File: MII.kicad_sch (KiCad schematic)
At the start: 2 parts, among them U2 ICE40HX8K-BG121

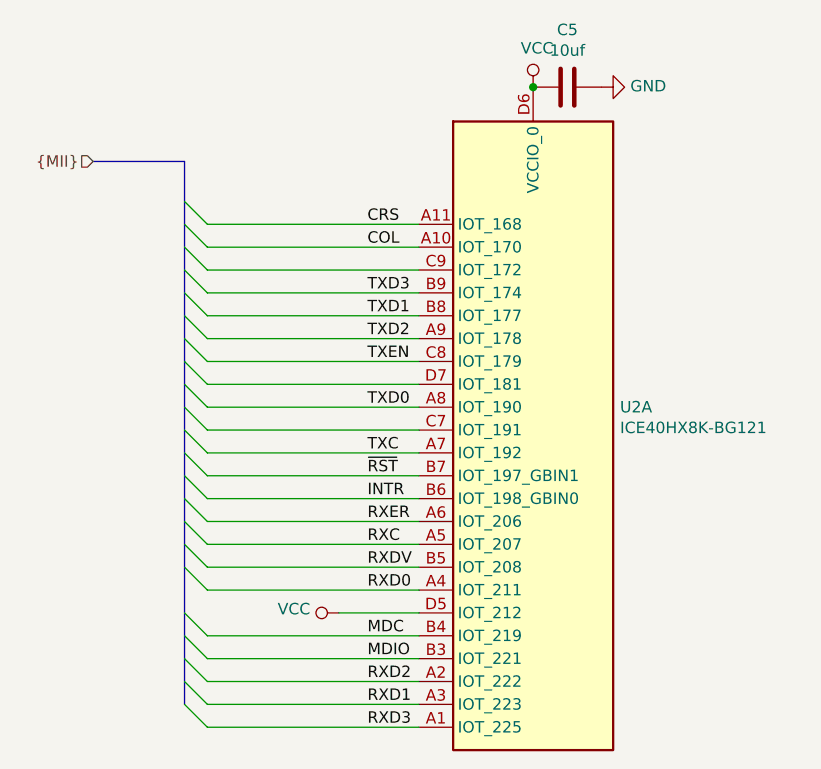
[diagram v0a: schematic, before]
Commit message: Routing changes, pullups, etc
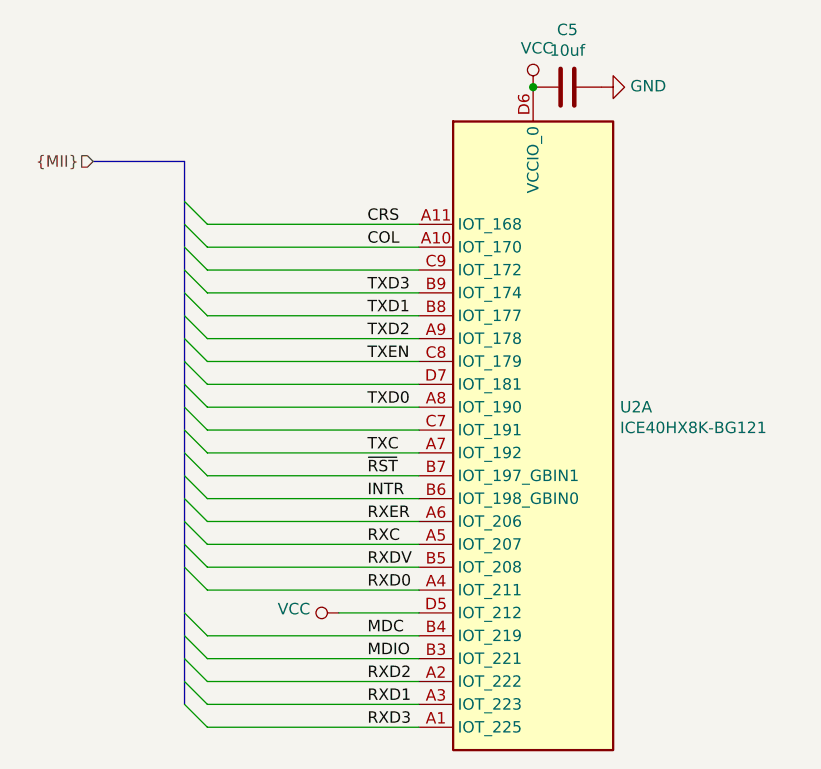
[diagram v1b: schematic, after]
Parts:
- C5, U2: Source (none) -> ANY
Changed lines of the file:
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@@
-(kicad_sch (version 20200512) (host eeschema "5.99.0-unknown-711fc99~101~ubuntu20.04.1")
-  (page 1 7)
+(kicad_sch (version 20200512) (host eeschema "5.99.0-unknown-eae0c14~101~ubuntu20.04.1")
+  (page 3 7)
   (paper "A4")
   (junction (at 111.125 62.23))
@@
   (bus_entry (at 72.39 128.27) (size 2.54 2.54))
   (bus_entry (at 72.39 130.81) (size 2.54 2.54))
-  (wire (pts (xy 74.93 77.47) (xy 98.425 77.47)))
-  (wire (pts (xy 74.93 80.01) (xy 98.425 80.01)))
-  (wire (pts (xy 74.93 82.55) (xy 98.425 82.55)))
-  (wire (pts (xy 74.93 85.09) (xy 98.425 85.09)))
-  (wire (pts (xy 74.93 87.63) (xy 98.425 87.63)))
-  (wire (pts (xy 74.93 90.17) (xy 98.425 90.17)))
-  (wire (pts (xy 74.93 92.71) (xy 98.425 92.71)))
-  (wire (pts (xy 74.93 95.25) (xy 98.425 95.25)))
-  (wire (pts (xy 74.93 97.79) (xy 98.425 97.79)))
-  (wire (pts (xy 74.93 100.33) (xy 98.425 100.33)))
-  (wire (pts (xy 74.93 102.87) (xy 98.425 102.87)))
-  (wire (pts (xy 74.93 105.41) (xy 98.425 105.41)))
-  (wire (pts (xy 74.93 107.95) (xy 98.425 107.95)))
-  (wire (pts (xy 74.93 110.49) (xy 98.425 110.49)))
-  (wire (pts (xy 74.93 113.03) (xy 98.425 113.03)))
-  (wire (pts (xy 74.93 115.57) (xy 98.425 115.57)))
-  (wire (pts (xy 74.93 118.11) (xy 98.425 118.11)))
-  (wire (pts (xy 74.93 123.19) (xy 98.425 123.19)))
-  (wire (pts (xy 74.93 125.73) (xy 98.425 125.73)))
-  (wire (pts (xy 74.93 128.27) (xy 98.425 128.27)))
-  (wire (pts (xy 74.93 130.81) (xy 98.425 130.81)))
-  (wire (pts (xy 74.93 133.35) (xy 98.425 133.35)))
-  (wire (pts (xy 89.535 120.65) (xy 98.425 120.65)))
-  (bus (pts (xy 62.23 70.485) (xy 72.39 70.485)))
-  (bus (pts (xy 72.39 70.485) (xy 72.39 77.47)))
-  (bus (pts (xy 72.39 77.47) (xy 72.39 82.55)))
-  (bus (pts (xy 72.39 82.55) (xy 72.39 87.63)))
-  (bus (pts (xy 72.39 87.63) (xy 72.39 92.71)))
-  (bus (pts (xy 72.39 92.71) (xy 72.39 97.79)))
-  (bus (pts (xy 72.39 97.79) (xy 72.39 102.87)))
-  (bus (pts (xy 72.39 102.87) (xy 72.39 107.95)))
-  (bus (pts (xy 72.39 107.95) (xy 72.39 110.49)))
-  (bus (pts (xy 72.39 110.49) (xy 72.39 115.57)))
-  (bus (pts (xy 72.39 115.57) (xy 72.39 120.65)))
-  (bus (pts (xy 72.39 120.65) (xy 72.39 125.73)))
-  (bus (pts (xy 72.39 125.73) (xy 72.39 130.81)))
+  (wire (pts (xy 74.93 77.47) (xy 98.425 77.47))
+    (stroke (width 0) (type solid) (color 0 0 0 0))
+  )
+  (wire (pts (xy 74.93 80.01) (xy 98.425 80.01))
+    (stroke (width 0) (type solid) (color 0 0 0 0))
+  )
+  (wire (pts (xy 74.93 82.55) (xy 98.425 82.55))
+    (stroke (width 0) (type solid) (color 0 0 0 0))
+  )
+  (wire (pts (xy 74.93 85.09) (xy 98.425 85.09))
+    (stroke (width 0) (type solid) (color 0 0 0 0))
+  )
+  (wire (pts (xy 74.93 87.63) (xy 98.425 87.63))
+    (stroke (width 0) (type solid) (color 0 0 0 0))
+  )
+  (wire (pts (xy 74.93 90.17) (xy 98.425 90.17))
+    (stroke (width 0) (type solid) (color 0 0 0 0))
+  )
+  (wire (pts (xy 74.93 92.71) (xy 98.425 92.71))
+    (stroke (width 0) (type solid) (color 0 0 0 0))
+  )
+  (wire (pts (xy 74.93 95.25) (xy 98.425 95.25))
+    (stroke (width 0) (type solid) (color 0 0 0 0))
+  )
+  (wire (pts (xy 74.93 97.79) (xy 98.425 97.79))
+    (stroke (width 0) (type solid) (color 0 0 0 0))
+  )
+  (wire (pts (xy 74.93 100.33) (xy 98.425 100.33))
+    (stroke (width 0) (type solid) (color 0 0 0 0))
+  )
+  (wire (pts (xy 74.93 102.87) (xy 98.425 102.87))
+    (stroke (width 0) (type solid) (color 0 0 0 0))
+  )
+  (wire (pts (xy 74.93 105.41) (xy 98.425 105.41))
+    (stroke (width 0) (type solid) (color 0 0 0 0))
+  )
+  (wire (pts (xy 74.93 107.95) (xy 98.425 107.95))
+    (stroke (width 0) (type solid) (color 0 0 0 0))
+  )
+  (wire (pts (xy 74.93 110.49) (xy 98.425 110.49))
+    (stroke (width 0) (type solid) (color 0 0 0 0))
+  )
+  (wire (pts (xy 74.93 113.03) (xy 98.425 113.03))
+    (stroke (width 0) (type solid) (color 0 0 0 0))
+  )
+  (wire (pts (xy 74.93 115.57) (xy 98.425 115.57))
+    (stroke (width 0) (type solid) (color 0 0 0 0))
+  )
+  (wire (pts (xy 74.93 118.11) (xy 98.425 118.11))
+    (stroke (width 0) (type solid) (color 0 0 0 0))
+  )
+  (wire (pts (xy 74.93 123.19) (xy 98.425 123.19))
+    (stroke (width 0) (type solid) (color 0 0 0 0))
+  )
+  (wire (pts (xy 74.93 125.73) (xy 98.425 125.73))
+    (stroke (width 0) (type solid) (color 0 0 0 0))
+  )
+  (wire (pts (xy 74.93 128.27) (xy 98.425 128.27))
+    (stroke (width 0) (type solid) (color 0 0 0 0))
+  )
+  (wire (pts (xy 74.93 130.81) (xy 98.425 130.81))
+    (stroke (width 0) (type solid) (color 0 0 0 0))
+  )
+  (wire (pts (xy 74.93 133.35) (xy 98.425 133.35))
+    (stroke (width 0) (type solid) (color 0 0 0 0))
+  )
+  (wire (pts (xy 89.535 120.65) (xy 98.425 120.65))
+    (stroke (width 0) (type solid) (color 0 0 0 0))
+  )
+  (bus (pts (xy 62.23 70.485) (xy 72.39 70.485))
+    (stroke (width 0) (type solid) (color 0 0 0 0))
+  )
+  (bus (pts (xy 72.39 70.485) (xy 72.39 77.47))
+    (stroke (width 0) (type solid) (color 0 0 0 0))
+  )
+  (bus (pts (xy 72.39 77.47) (xy 72.39 82.55))
+    (stroke (width 0) (type solid) (color 0 0 0 0))
+  )
+  (bus (pts (xy 72.39 82.55) (xy 72.39 87.63))
+    (stroke (width 0) (type solid) (color 0 0 0 0))
+  )
+  (bus (pts (xy 72.39 87.63) (xy 72.39 92.71))
+    (stroke (width 0) (type solid) (color 0 0 0 0))
+  )
+  (bus (pts (xy 72.39 92.71) (xy 72.39 97.79))
+    (stroke (width 0) (type solid) (color 0 0 0 0))
+  )
+  (bus (pts (xy 72.39 97.79) (xy 72.39 102.87))
+    (stroke (width 0) (type solid) (color 0 0 0 0))
+  )
+  (bus (pts (xy 72.39 102.87) (xy 72.39 105.41))
+    (stroke (width 0) (type solid) (color 0 0 0 0))
+  )
+  (bus (pts (xy 72.39 105.41) (xy 72.39 110.49))
+    (stroke (width 0) (type solid) (color 0 0 0 0))
+  )
+  (bus (pts (xy 72.39 110.49) (xy 72.39 115.57))
+    (stroke (width 0) (type solid) (color 0 0 0 0))
+  )
+  (bus (pts (xy 72.39 115.57) (xy 72.39 120.65))
+    (stroke (width 0) (type solid) (color 0 0 0 0))
+  )
+  (bus (pts (xy 72.39 120.65) (xy 72.39 125.73))
+    (stroke (width 0) (type solid) (color 0 0 0 0))
+  )
+  (bus (pts (xy 72.39 125.73) (xy 72.39 130.81))
+    (stroke (width 0) (type solid) (color 0 0 0 0))
+  )
   (label "CRS" (at 92.71 77.47 0)
     (effects (font (size 1.27 1.27)) (justify left bottom))
@@
       (effects (font (size 1.27 1.27)) hide)
     )
+    (property "Source" "ANY" (id 4) (at 114.935 62.23 0)
+      (effects (font (size 1.27 1.27)) hide)
+    )
   )
   (symbol (lib_id "FPGA_Lattice:ICE40HX8K-BG121") (at 111.125 97.79 0) (unit 1)
@@
       (effects (font (size 1.27 1.27)) hide)
     )
+    (property "Source" "ANY" (id 4) (at 111.125 97.79 0)
+      (effects (font (size 1.27 1.27)) hide)
+    )
